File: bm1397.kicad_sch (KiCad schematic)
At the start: 32 parts, among them IC1 BM1397_mode1, Q1 2N7002, U2 25MHz, U3 MCP1824T-1802E, U4 MCP1824T-0802E, U6 TXU0202DCUR

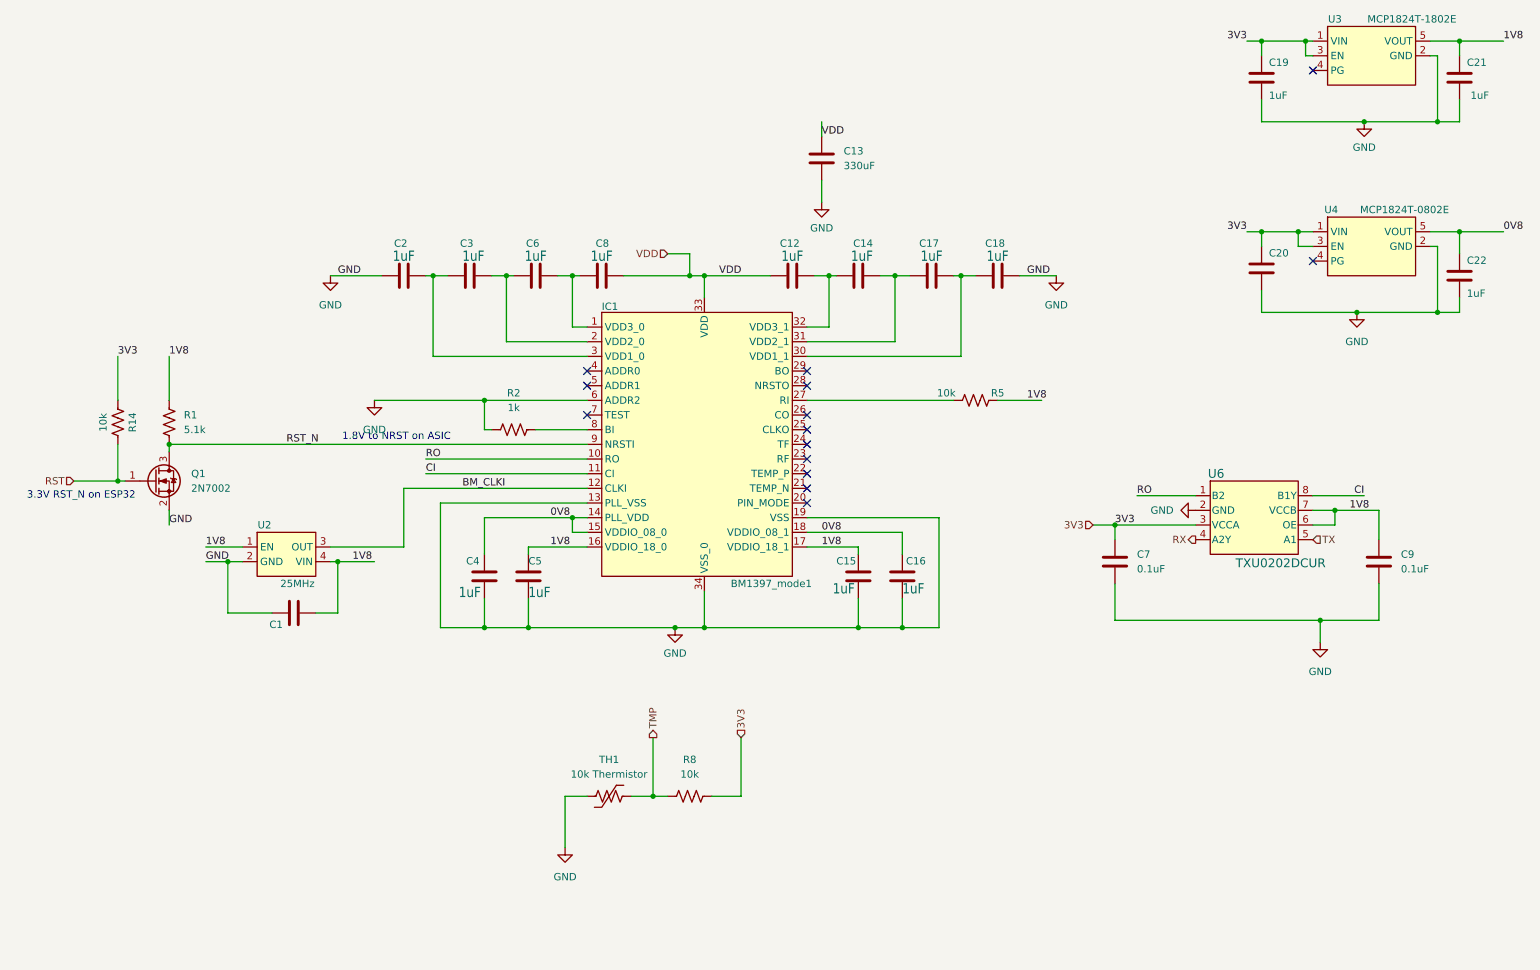
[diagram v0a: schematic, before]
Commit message: BM1366
BM1366 tryout
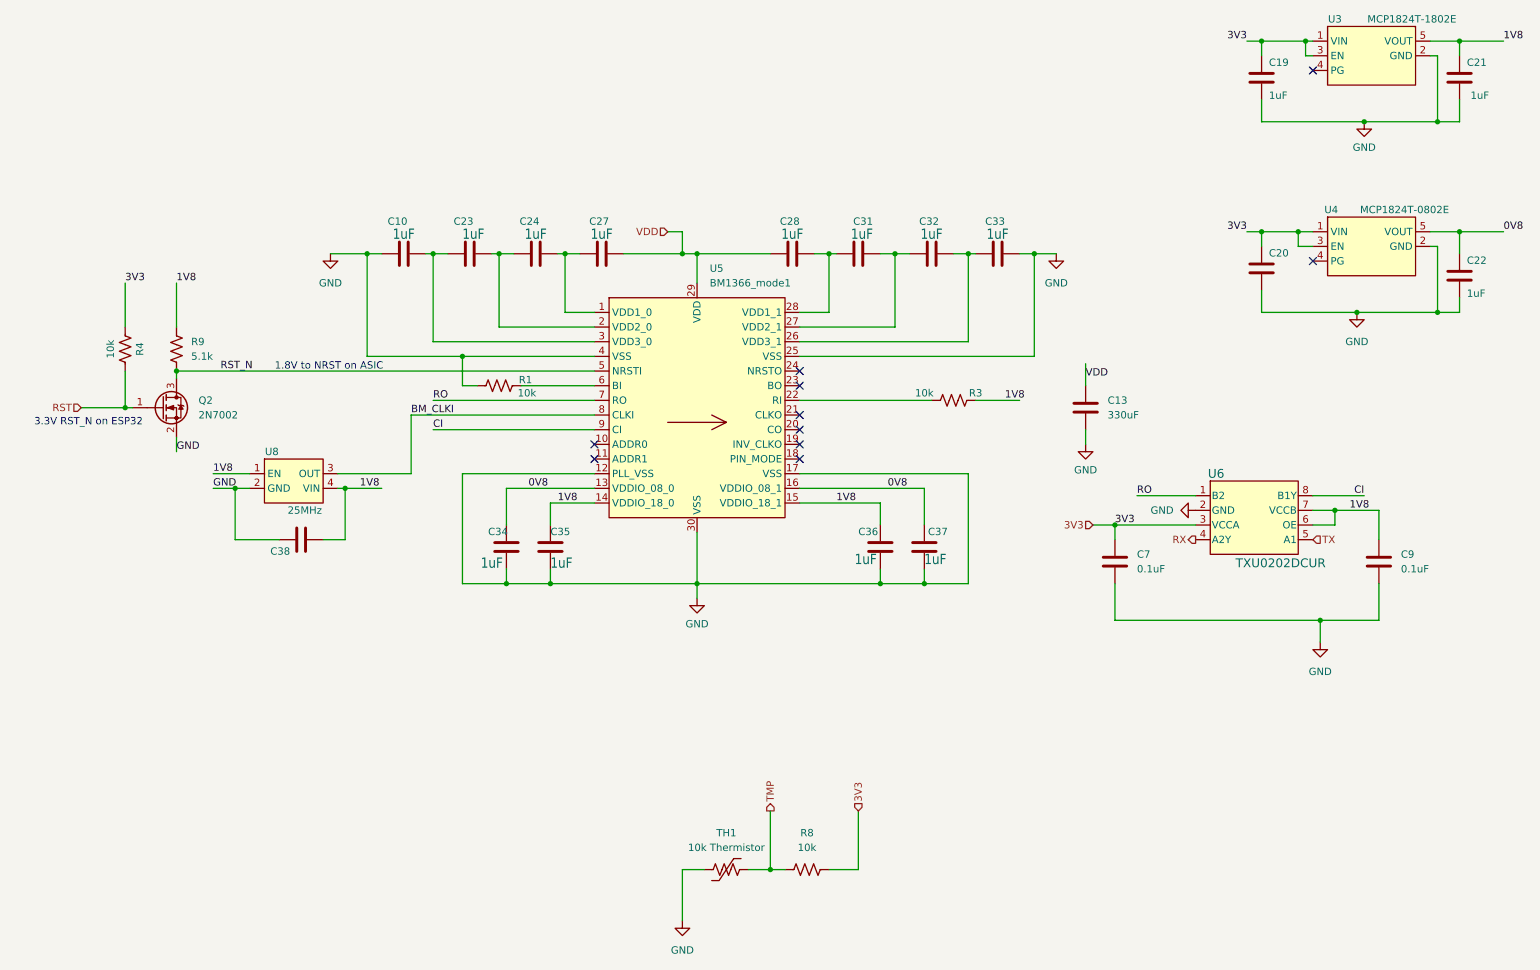
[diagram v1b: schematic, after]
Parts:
- removed C1: 0.1uF, Capacitor_SMD:C_0402_1005Metric, symbol Device:C
- removed C12, C14, C15, C16, C17, C18, C2, C3, C4, C5, C6, C8: 1uF, Capacitor_SMD:C_0402_1005Metric, symbol Device:C
- removed IC1: BM1397_mode1, bitaxe:BM1397, symbol bitaxe:BM1397_mode1
- removed Q1: 2N7002, Package_TO_SOT_SMD:SOT-23, symbol Transistor_FET:2N7002
- removed R14, R5: 10k, Resistor_SMD:R_0402_1005Metric, symbol Device:R_US
- removed R2: 1k, Resistor_SMD:R_0402_1005Metric, symbol Device:R_US
- removed U2: 25MHz, bitaxe:O 25,0-JO32-B-1V3-1-T1-LF, symbol bitaxe:oscillator
- added C10, C23, C24, C27, C28, C31, C32, C33, C34, C35, C36, C37: 1uF, Capacitor_SMD:C_0402_1005Metric, symbol Device:C
- added C38: 0.1uF, Capacitor_SMD:C_0402_1005Metric, symbol Device:C
- added Q2: 2N7002, Package_TO_SOT_SMD:SOT-23, symbol Transistor_FET:2N7002
- added R3, R4: 10k, Resistor_SMD:R_0402_1005Metric, symbol Device:R_US
- added R9: 5.1k, Resistor_SMD:R_0402_1005Metric, symbol Device:R_US
- added U5: BM1366_mode1, bitaxe:BM1366, symbol bitaxe:BM1366_mode1
- added U8: 25MHz, bitaxe:O 25,0-JO32-B-1V3-1-T1-LF, symbol bitaxe:oscillator
- R1: value 5.1k -> 10k; footprint Resistor_SMD:R_0402_1005Metric -> PCM_Resistor_SMD_AKL:R_0402_1005Metric; DK RMCF0402JT5K10CT-ND -> (none); PARTNO ERJ-2RKF2491X -> (none)
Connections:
- net 0V8: now also C34.1, C37.1, U5.13 (VDDIO_08_0), U5.16 (VDDIO_08_1)
- net 1V8: now also C35.1, C36.1, C38.2, R3.2, R9.2, U5.14 (VDDIO_18_0), U5.15 (VDDIO_18_1), U8.1 (EN), U8.4 (VIN); no longer R1.2
- net 3V3: now also R4.1
- net BM_CLKI: now also U5.8 (CLKI), U8.3 (OUT)
- net CI: now also U5.9 (CI)
- net GND: now also R1.1, C10.1, C33.2, C34.2, C35.2, C36.2, C37.2, C38.1, Q2.2 (S), U5.12 (PLL_VSS), U5.17 (VSS), U5.25 (VSS), U5.30 (VSS), U5.4 (VSS), U8.2 (GND)
- net RO: now also U5.7 (RO)
- net RST: now also Q2.1 (G), R4.2
- net RST_N: now also Q2.3 (D), R9.1, U5.5 (NRSTI); no longer R1.1
- net VDD: now also C27.2, C28.1, U5.29 (VDD)
- new net: C23.2, C24.1, U5.2 (VDD2_0)
- new net: C24.2, C27.1, U5.1 (VDD1_0)
- new net: R1.2, U5.6 (BI)
- new net: R3.1, U5.22 (RI)
- new net: C32.2, C33.1, U5.26 (VDD3_1)
- new net: C31.2, C32.1, U5.27 (VDD2_1)
- new net: C28.2, C31.1, U5.28 (VDD1_1)
- new net: C10.2, C23.1, U5.3 (VDD3_0)
- no-connect marks 14 -> 10
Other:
- moved on the sheet: C13, R8, TH1
